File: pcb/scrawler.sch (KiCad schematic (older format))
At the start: 24 parts, among them SW1 switch, SW10 switch, SW11 switch, SW12 switch, SW13 switch, SW14 switch, SW15 switch, SW16 switch, SW17 switch, SW18 switch, SW19 switch, SW2 switch, SW20 switch, SW21 switch, SW22 switch, SW23 switch, SW3 switch, SW4 switch, SW5 switch, SW6 switch, SW7 switch, SW8 switch, SW9 switch

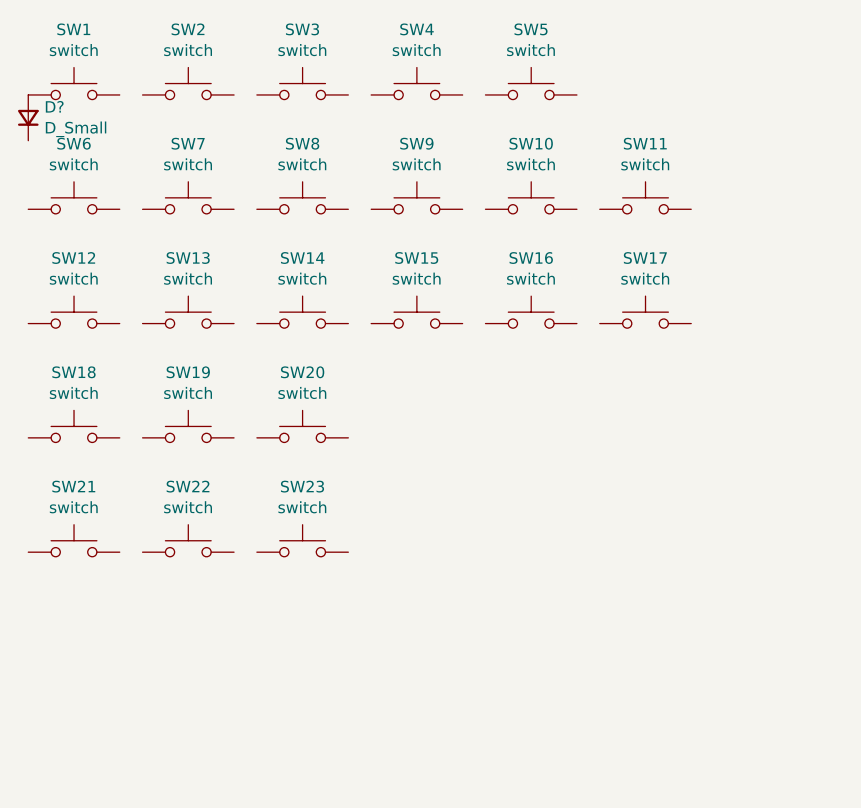
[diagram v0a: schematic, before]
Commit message: laptop commit
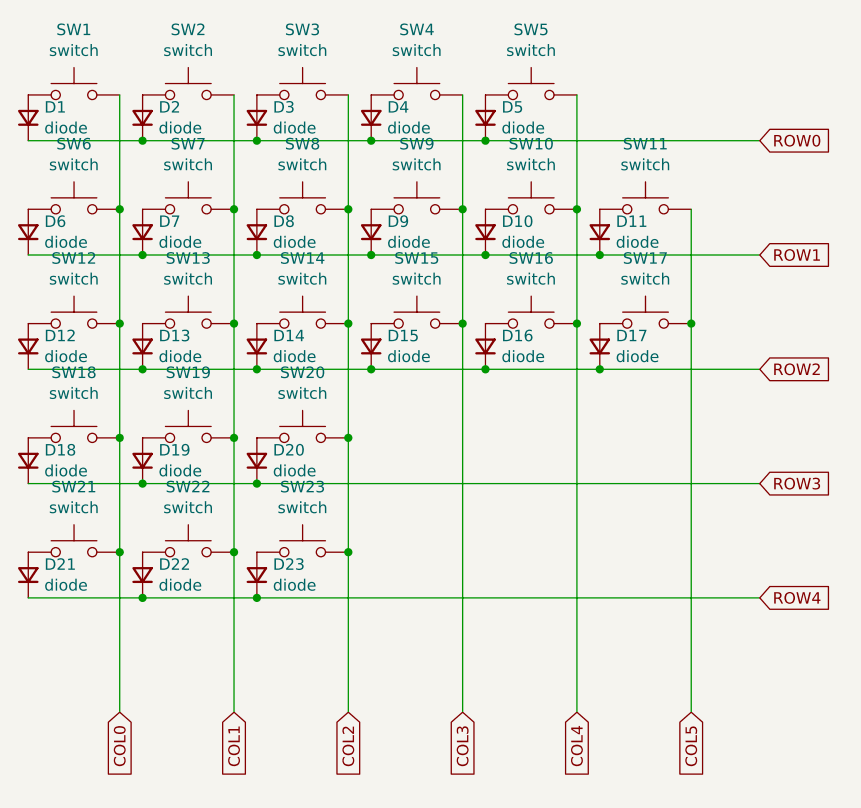
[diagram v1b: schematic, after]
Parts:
- added D10, D11, D12, D13, D14, D15, D16, D17, D18, D19, D2, D20, D21, D22, D23, D3, D4, D5, D6, D7, D8, D9: diode, symbol Device:D_Small
- D1: renamed from D?; value D_Small -> diode
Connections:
- net COL0: now reaches SW1.2
- net COL0: now also SW12.2, SW18.2, SW21.2, SW6.2
- net at SW2.1: now also D2.2 (A)
- net COL1: now reaches SW2.2
- net COL1: now also SW13.2, SW19.2, SW22.2, SW7.2
- net at SW3.1: now also D3.2 (A)
- net COL2: now reaches SW3.2
- net COL2: now also SW14.2, SW20.2, SW23.2, SW8.2
- net at SW4.1: now also D4.2 (A)
- net COL3: now reaches SW4.2
- net COL3: now also SW15.2, SW9.2
- net at SW5.1: now also D5.2 (A)
- net COL4: now reaches SW5.2
- net COL4: now also SW10.2, SW16.2
- net at SW6.1: now also D6.2 (A)
- net at SW7.1: now also D7.2 (A)
- net at SW8.1: now also D8.2 (A)
- net at SW9.1: now also D9.2 (A)
- net at SW10.1: now also D10.2 (A)
- net at SW12.1: now also D12.2 (A)
- net at SW13.1: now also D13.2 (A)
- net at SW14.1: now also D14.2 (A)
- net at SW15.1: now also D15.2 (A)
- net at SW16.1: now also D16.2 (A)
- net at SW11.1: now also D11.2 (A)
- net COL5: now reaches SW11.2
- net COL5: now also SW17.2
- net at SW17.1: now also D17.2 (A)
- net at SW18.1: now also D18.2 (A)
- net at SW19.1: now also D19.2 (A)
- net at SW20.1: now also D20.2 (A)
- net at SW21.1: now also D21.2 (A)
- net at SW22.1: now also D22.2 (A)
- net at SW23.1: now also D23.2 (A)
- net ROW0: now reaches D1.1 (K)
- net ROW0: now also D2.1 (K), D3.1 (K), D4.1 (K), D5.1 (K)
- new net ROW1: D10.1 (K), D11.1 (K), D6.1 (K), D7.1 (K), D8.1 (K), D9.1 (K)
- new net ROW2: D12.1 (K), D13.1 (K), D14.1 (K), D15.1 (K), D16.1 (K), D17.1 (K)
- new net ROW3: D18.1 (K), D19.1 (K), D20.1 (K)
- new net ROW4: D21.1 (K), D22.1 (K), D23.1 (K)
